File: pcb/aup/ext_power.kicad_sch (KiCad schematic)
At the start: 28 parts, among them J5 Conn_01x02_Pin, Q1 AO3401A, U10 TPS2116DRLR, U2 USBLC6-2SC6, U3 TPS563257DRLR

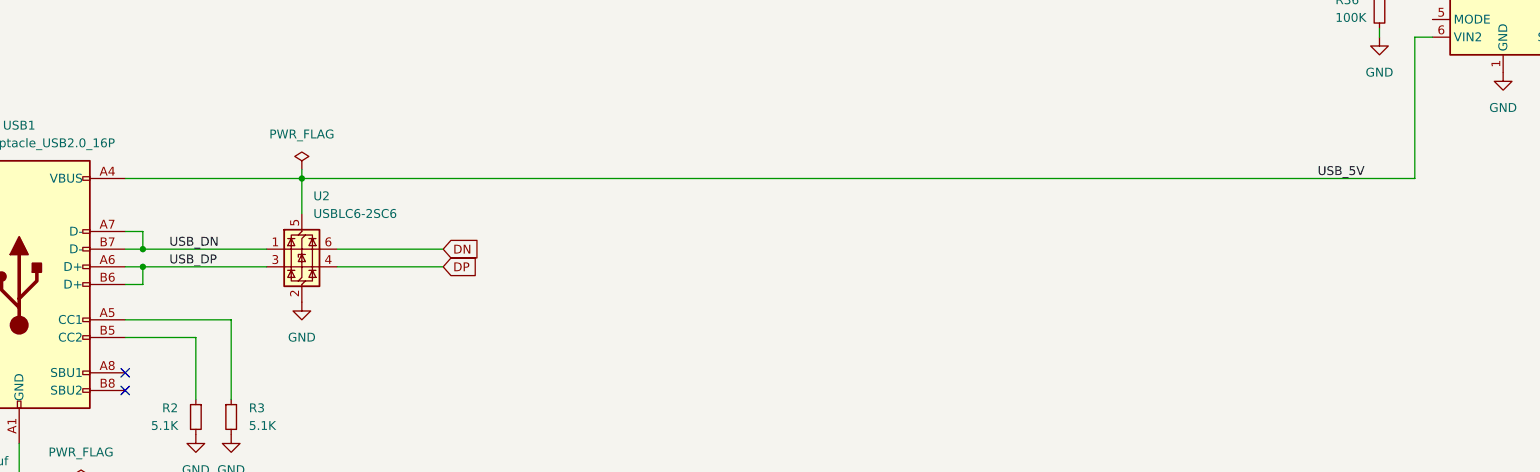
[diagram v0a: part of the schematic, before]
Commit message: Start of regulator rework
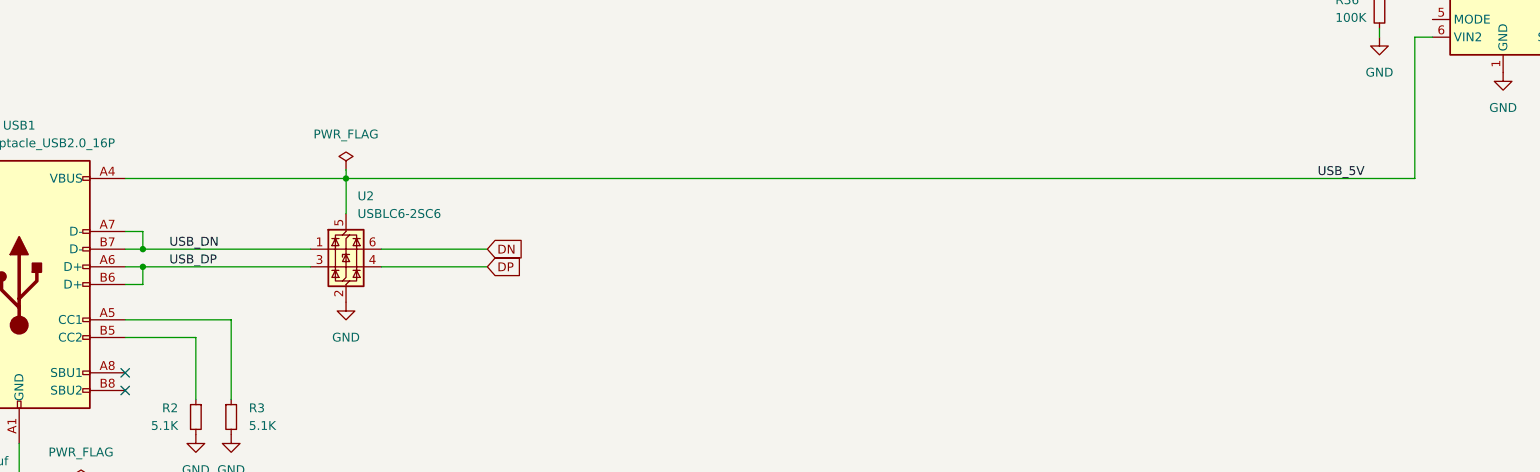
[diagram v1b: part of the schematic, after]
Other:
- moved on the sheet: U2
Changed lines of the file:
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@@
 	)
 	(junction
-		(at 73.66 111.76)
+		(at 80.01 111.76)
 		(diameter 0)
 		(color 0 0 0 0)
@@
 	(wire
 		(pts
-			(xy 73.66 111.76) (xy 73.66 116.84)
+			(xy 80.01 111.76) (xy 80.01 116.84)
 		)
 		(stroke
@@
 	(wire
 		(pts
-			(xy 48.26 111.76) (xy 73.66 111.76)
+			(xy 48.26 111.76) (xy 80.01 111.76)
 		)
 		(stroke
@@
 	(wire
 		(pts
-			(xy 73.66 111.76) (xy 73.66 110.49)
+			(xy 80.01 111.76) (xy 80.01 110.49)
 		)
 		(stroke
@@
 	(wire
 		(pts
-			(xy 50.8 124.46) (xy 68.58 124.46)
+			(xy 50.8 124.46) (xy 74.93 124.46)
 		)
 		(stroke
@@
 	(wire
 		(pts
-			(xy 78.74 124.46) (xy 93.98 124.46)
+			(xy 85.09 124.46) (xy 100.33 124.46)
 		)
 		(stroke
@@
 	(wire
 		(pts
-			(xy 50.8 121.92) (xy 68.58 121.92)
+			(xy 50.8 121.92) (xy 74.93 121.92)
 		)
 		(stroke
@@
 	(wire
 		(pts
+			(xy 80.01 111.76) (xy 233.68 111.76)
+		)
+		(stroke
+			(width 0)
+			(type default)
+		)
+	)
+	(wire
+		(pts
 			(xy 247.65 44.45) (xy 245.11 44.45)
 		)
@@
 	(wire
 		(pts
-			(xy 73.66 111.76) (xy 233.68 111.76)
-		)
-		(stroke
-			(width 0)
-			(type default)
-		)
-	)
-	(wire
-		(pts
 			(xy 31.75 156.21) (xy 33.02 156.21)
 		)
@@
 	(wire
 		(pts
-			(xy 78.74 121.92) (xy 93.98 121.92)
+			(xy 85.09 121.92) (xy 100.33 121.92)
 		)
 		(stroke
@@
 	(global_label "DP"
 		(shape input)
-		(at 93.98 124.46 0)
+		(at 100.33 124.46 0)
 		(fields_autoplaced yes)
 		(effects
@@
 		)
 		(property "Intersheetrefs" "${INTERSHEET_REFS}"
-			(at 99.5052 124.46 0)
+			(at 105.8552 124.46 0)
 			(effects
 				(font
@@
 	(global_label "DN"
 		(shape input)
-		(at 93.98 121.92 0)
+		(at 100.33 121.92 0)
 		(fields_autoplaced yes)
 		(effects
@@
 		)
 		(property "Intersheetrefs" "${INTERSHEET_REFS}"
-			(at 99.5657 121.92 0)
+			(at 105.9157 121.92 0)
 			(effects
 				(font
@@
 	(symbol
 		(lib_id "power:GND")
-		(at 73.66 129.54 0)
+		(at 80.01 129.54 0)
 		(unit 1)
 		(exclude_from_sim no)
@@
 		(fields_autoplaced yes)
 		(property "Reference" "#PWR06"
-			(at 73.66 135.89 0)
+			(at 80.01 135.89 0)
 			(effects
 				(font
@@
 		)
 		(property "Value" "GND"
-			(at 73.66 134.62 0)
+			(at 80.01 134.62 0)
 			(effects
 				(font
@@
 		)
 		(property "Footprint" ""
-			(at 73.66 129.54 0)
+			(at 80.01 129.54 0)
 			(effects
 				(font
@@
 		)
 		(property "Datasheet" ""
-			(at 73.66 129.54 0)
+			(at 80.01 129.54 0)
 			(effects
 				(font
@@
 		)
 		(property "Description" "Power symbol creates a global label with name \"GND\" , ground"
-			(at 73.66 129.54 0)
+			(at 80.01 129.54 0)
 			(effects
 				(font
@@
 	(symbol
 		(lib_id "!Misc:USBLC6-2SC6")
-		(at 73.66 121.92 0)
+		(at 80.01 121.92 0)
 		(unit 1)
 		(exclude_from_sim no)
@@
 		(fields_autoplaced yes)
 		(property "Reference" "U2"
-			(at 75.3111 114.3 0)
+			(at 81.6611 114.3 0)
 			(effects
 				(font
@@
 		)
 		(property "Value" "USBLC6-2SC6"
-			(at 75.3111 116.84 0)
+			(at 81.6611 116.84 0)
 			(effects
 				(font
@@
 		)
 		(property "Footprint" "Package_TO_SOT_SMD:SOT-23-6"
-			(at 74.93 128.27 0)
+			(at 81.28 128.27 0)
 			(effects
 				(font
@@
 		)
 		(property "Datasheet" "https://www.st.com/resource/en/datasheet/usblc6-2.pdf"
-			(at 74.93 130.175 0)
+			(at 81.28 130.175 0)
 			(effects
 				(font
@@
 		)
 		(property "Description" "Very low capacitance ESD protection diode, 2 data-line, SOT-23-6"
-			(at 73.66 121.92 0)
+			(at 80.01 121.92 0)
 			(effects
 				(font
@@
 		)
 		(property "LCSC Part #" "C7519"
-			(at 73.66 121.92 0)
+			(at 80.01 121.92 0)
 			(effects
 				(font
@@
 		)
 		(property "Digi-Key Part Number" "497-5235-1-ND"
-			(at 73.66 121.92 0)
+			(at 80.01 121.92 0)
 			(effects
 				(font
@@
 	(symbol
 		(lib_id "power:PWR_FLAG")
-		(at 73.66 110.49 0)
+		(at 80.01 110.49 0)
 		(unit 1)
 		(exclude_from_sim no)
@@
 		(dnp no)
 		(property "Reference" "#FLG02"
-			(at 73.66 108.585 0)
+			(at 80.01 108.585 0)
 			(effects
 				(font
@@
 		)
 		(property "Value" "PWR_FLAG"
-			(at 73.66 105.41 0)
+			(at 80.01 105.41 0)
 			(effects
 				(font
@@
 		)
 		(property "Footprint" ""
-			(at 73.66 110.49 0)
+			(at 80.01 110.49 0)
 			(effects
 				(font
@@
 		)
 		(property "Datasheet" "~"
-			(at 73.66 110.49 0)
+			(at 80.01 110.49 0)
 			(effects
 				(font
@@
 		)
 		(property "Description" "Special symbol for telling ERC where power comes from"
-			(at 73.66 110.49 0)
+			(at 80.01 110.49 0)
 			(effects
 				(font
